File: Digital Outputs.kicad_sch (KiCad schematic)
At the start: 18 parts, among them J10 Screw_Terminal_01x06, J11 Screw_Terminal_01x06, J12 Screw_Terminal_01x06, J9 Screw_Terminal_01x06, K1 HF46F-G, K10 HF46F-G, K11 HF46F-G, K12 HF46F-G, K2 HF46F-G, K3 HF46F-G, K4 HF46F-G, K5 HF46F-G, K6 HF46F-G, K7 HF46F-G, K8 HF46F-G, K9 HF46F-G, U1 ULN2003, U12 ULN2003

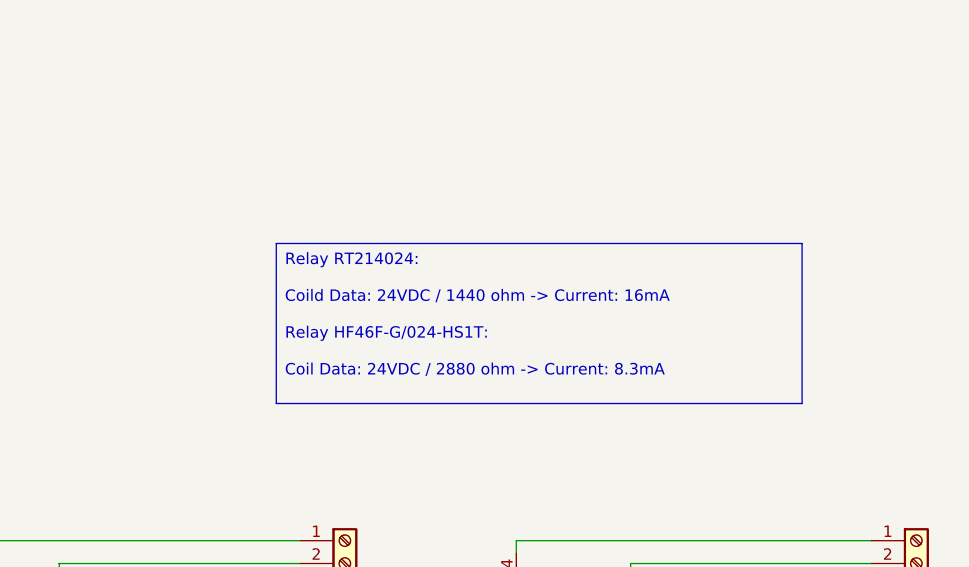
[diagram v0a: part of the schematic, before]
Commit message: Avance
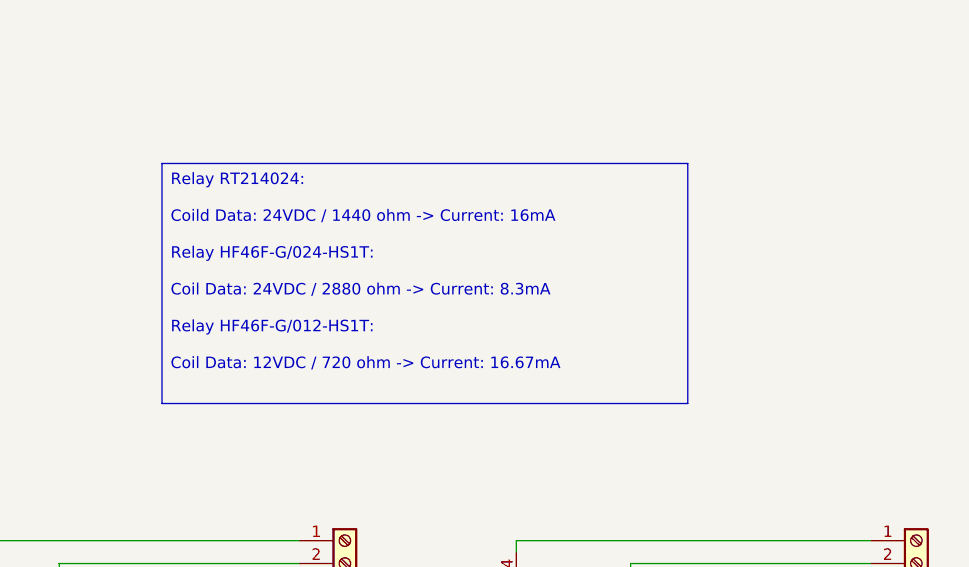
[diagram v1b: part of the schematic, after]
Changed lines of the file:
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@@
 		)
 	)
-	(text_box "Relay RT214024:\n\nCoild Data: 24VDC / 1440 ohm -> Current: 16mA\n\nRelay HF46F-G/024-HS1T:\n\nCoil Data: 24VDC / 2880 ohm -> Current: 8.3mA"
+	(text_box "Relay RT214024:\n\nCoild Data: 24VDC / 1440 ohm -> Current: 16mA\n\nRelay HF46F-G/024-HS1T:\n\nCoil Data: 24VDC / 2880 ohm -> Current: 8.3mA\n\nRelay HF46F-G/012-HS1T:\n\nCoil Data: 12VDC / 720 ohm -> Current: 16.67mA"
 		(exclude_from_sim no)
-		(at 290.83 63.5 0)
-		(size 58.42 17.78)
+		(at 278.13 54.61 0)
+		(size 58.42 26.67)
 		(margins 0.9525 0.9525 0.9525 0.9525)
 		(stroke
